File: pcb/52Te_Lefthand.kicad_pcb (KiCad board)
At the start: 2 copper layers, 55 parts, among them J1 MJ-4PP-9, SW1 SW_PUSH, SW10 SW_PUSH, SW11 SW_PUSH, SW12 SW_PUSH, SW13 SW_PUSH, SW14 SW_PUSH, SW15 SW_PUSH, SW16 SW_PUSH, SW17 SW_PUSH, SW18 SW_PUSH, SW19 SW_PUSH, SW2 SW_PUSH, SW20 SW_PUSH, SW21 SW_PUSH, SW22 SW_PUSH, SW23 SW_PUSH, SW24 SW_PUSH, SW25 SW_PUSH, SW26 SW_PUSH, SW27 SW_PUSH, SW3 SW_PUSH, SW4 SW_PUSH, SW5 SW_PUSH, SW6 SW_PUSH, SW7 SW_PUSH, SW8 SW_PUSH, SW9 SW_PUSH, U1 ProMicro

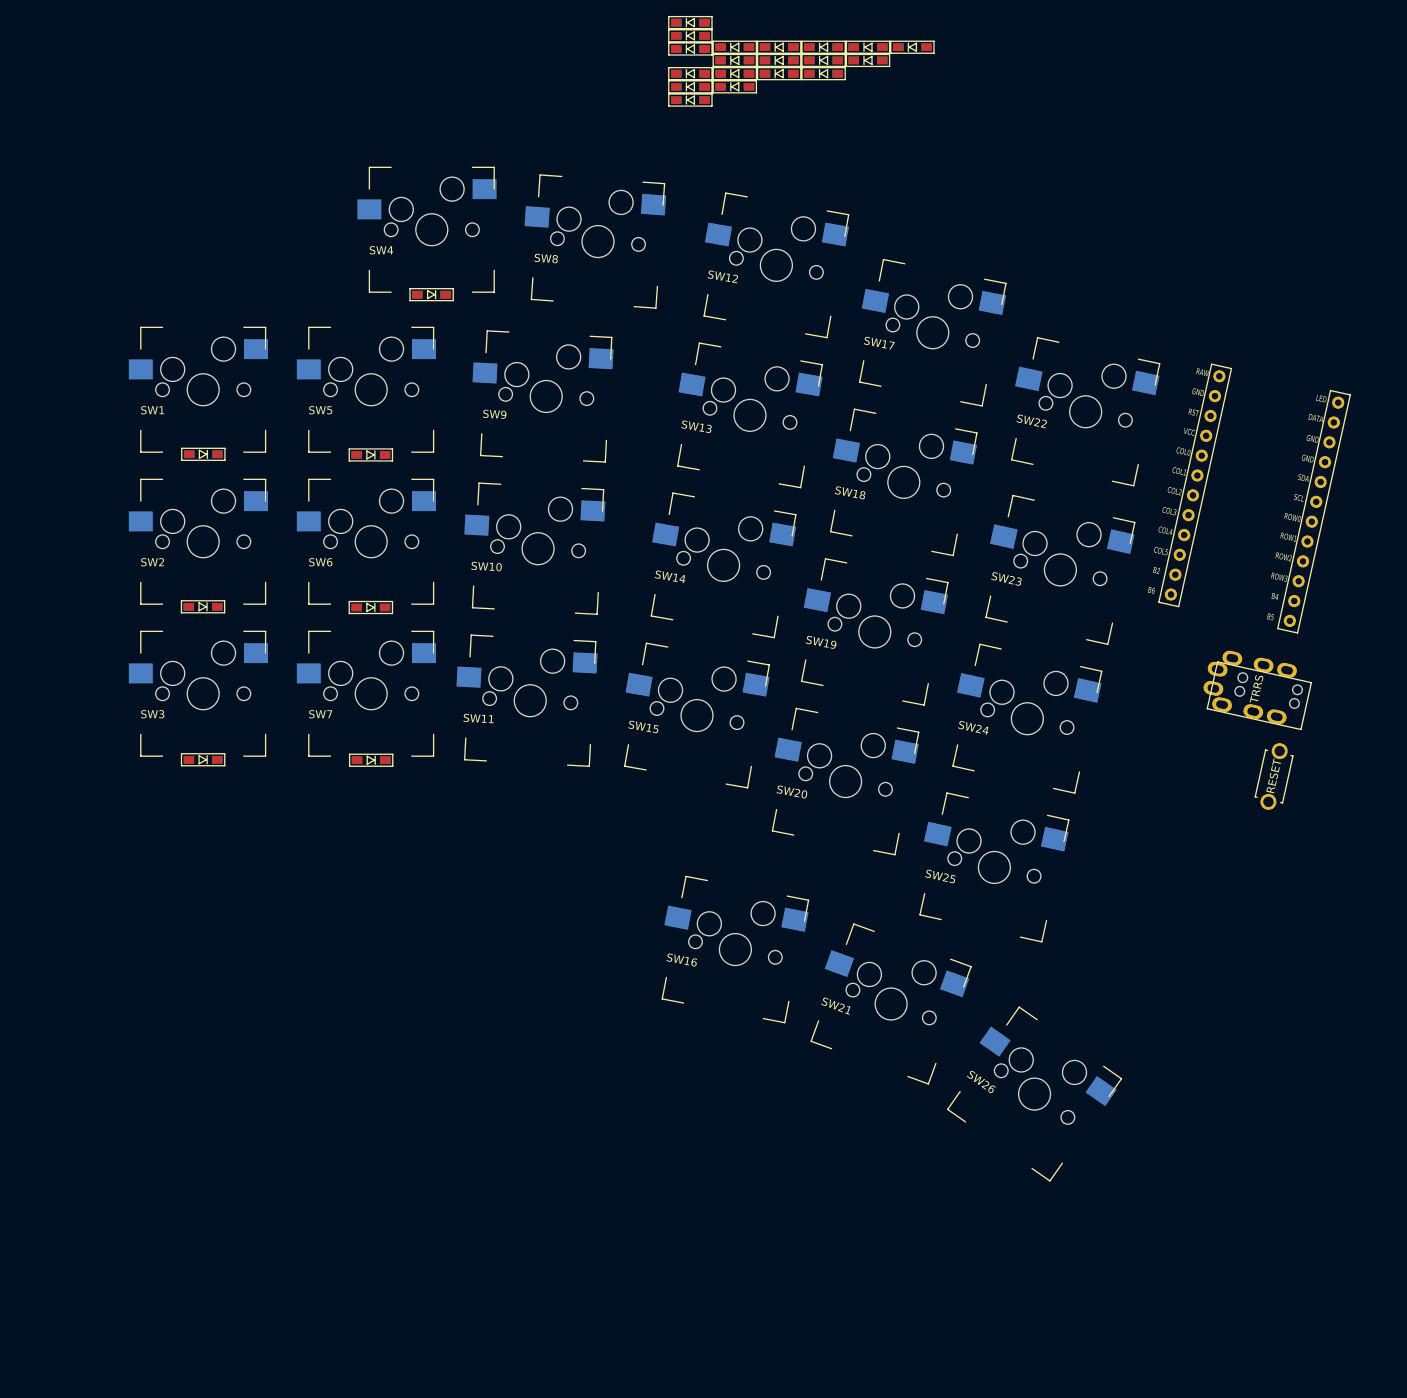
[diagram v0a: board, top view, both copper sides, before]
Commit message: first draft pcb lefthand
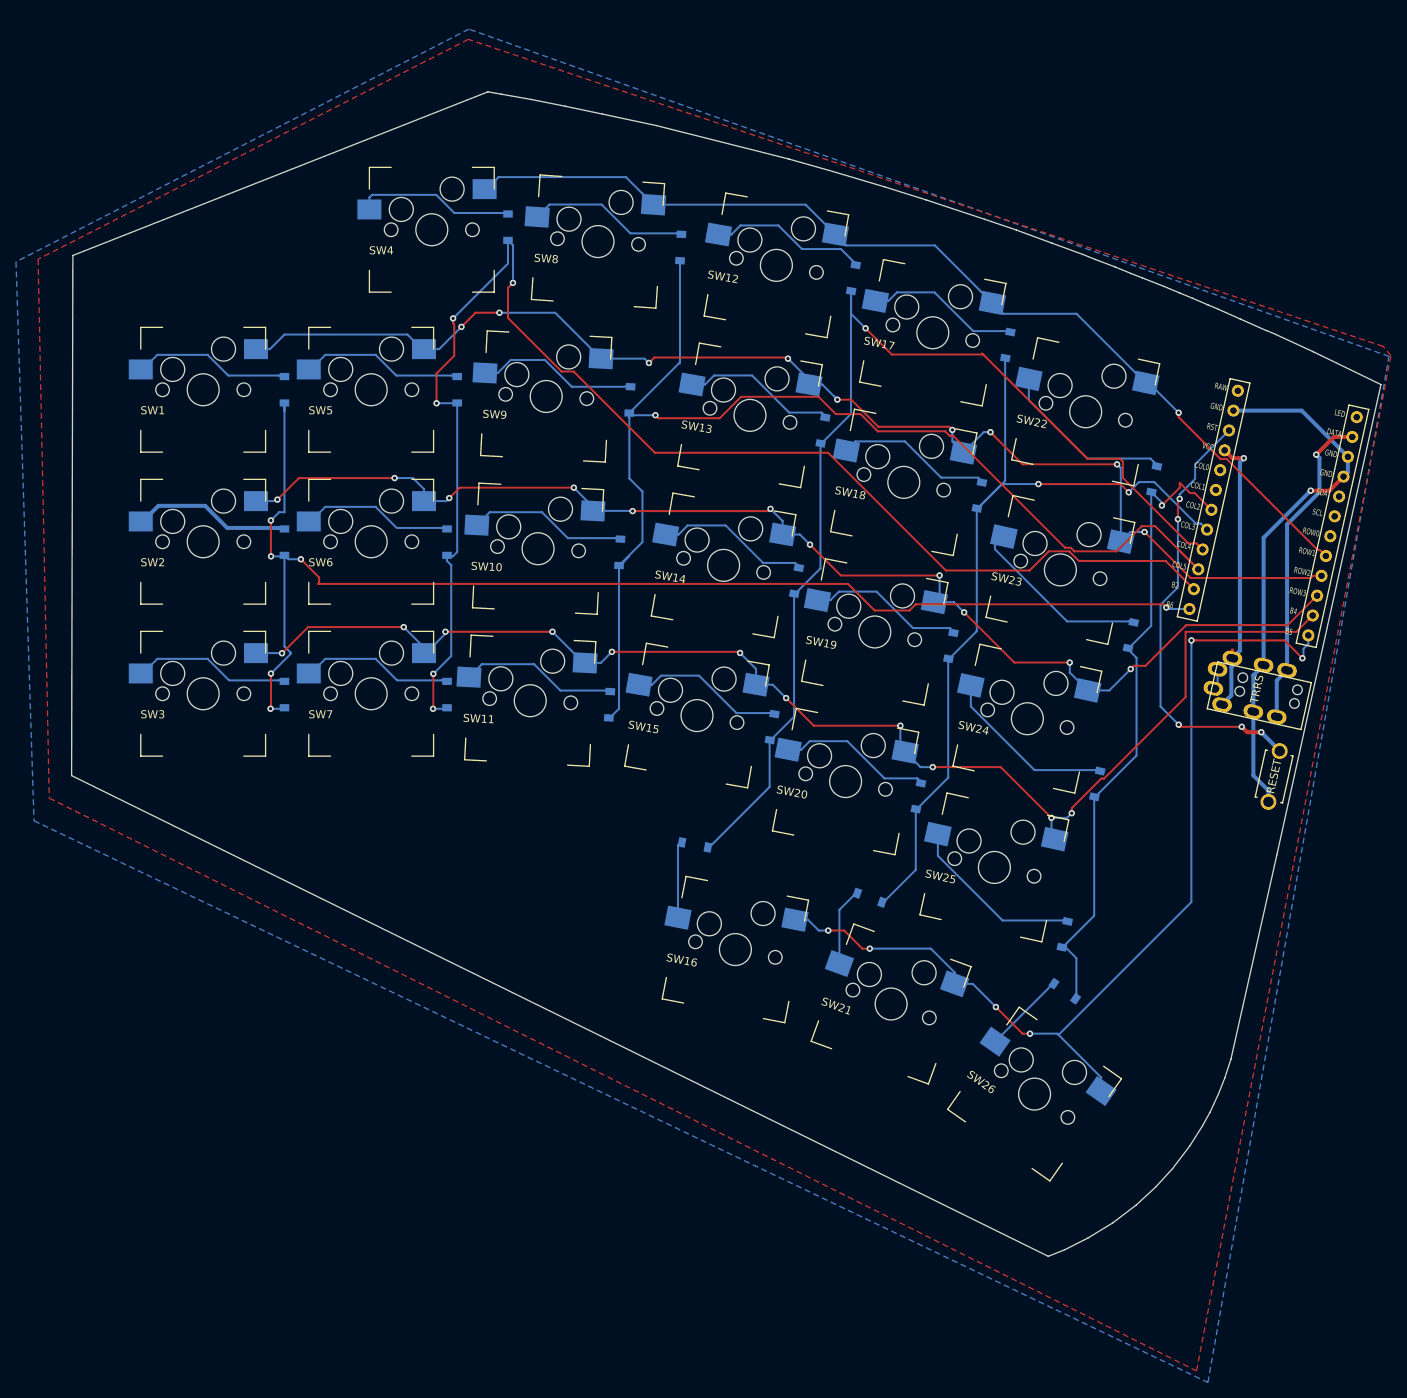
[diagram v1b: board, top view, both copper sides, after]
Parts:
- D1, D2, D3, D4, D5, D6, D7: footprint kbd:D3_SMD -> Diode_SMD:D_SOD-123
- D10, D11, D12, D13, D14, D15, D16, D17, D18, D19, D20, D21, D22, D23, D24, D25, D26, D8, D9: footprint kbd:D3_SMD -> Diode_SMD:D_SOD-123; moved to B.Cu
- moved D26 128.3 mm to (312.3, 188.2), turned to 145 degrees
- moved D25 120.2 mm to (312.3, 181.1), turned to 77.5 degrees
- moved D21 104.4 mm to (287.9, 176.5), turned to 160 degrees
- moved D24 102.6 mm to (316.4, 162.3), turned to 77.5 degrees
- moved D16 98.6 mm to (266.1, 169.9), turned to 169 degrees
- moved D20 93.1 mm to (294.0, 163.8), turned to 79 degrees
- moved D11 90.5 mm to (255.4, 152.4), turned to 87 degrees
- moved D15 88.7 mm to (275.7, 155.2), turned to 80 degrees
- moved D23 87.3 mm to (320.6, 143.7), turned to 77.5 degrees
- moved D22 77.0 mm to (323.5, 124.2), turned to 78 degrees
- moved D19 75.6 mm to (298.1, 145.0), turned to 79 degrees
- moved D10 66.6 mm to (256.7, 133.3), turned to 87 degrees
- moved D14 63.4 mm to (278.8, 136.9), turned to 80 degrees
- moved D18 59.5 mm to (301.7, 126.2), turned to 79 degrees
- moved D9 51.8 mm to (258.0, 114.3), turned to 87 degrees
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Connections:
- net +5V renamed GND
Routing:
- net col1: track 0.00 -> 180.9 mm, vias 0 -> 5
- net row3: track 0.00 -> 168.4 mm, vias 0 -> 11
- net col0: track 0.00 -> 162.3 mm, vias 0 -> 6
- net row1: track 0.00 -> 160.7 mm, vias 0 -> 9
- net row2: track 0.00 -> 157.1 mm, vias 0 -> 11
- net col2: track 0.00 -> 151.2 mm, vias 0 -> 1
- net col3: track 0.00 -> 137.2 mm, vias 0 -> 1
- net row0: track 0.00 -> 125.7 mm, vias 0 -> 1
- net row4: track 0.00 -> 123.1 mm, vias 0 -> 6
- net col4: track 0.00 -> 107.8 mm, vias 0 -> 2
- net col5: track 0.00 -> 81.3 mm, vias 0 -> 1
- net GND: track 0.00 -> 66.9 mm, vias 0 -> 1
- net reset: track 0.00 -> 55.3 mm, vias 0 -> 5
- net data: track 0.00 -> 40.6 mm, vias 0 -> 1
- net VCC: track 0.00 -> 35.9 mm, vias 0 -> 1
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- added copper zone on B.Cu, net GND
- added copper zone on F.Cu, net GND
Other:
- board outline added: 163.7 x 145.6 mm
- board text added: "52Te v1.0 PCB designed by @SA_EndlessGame"
